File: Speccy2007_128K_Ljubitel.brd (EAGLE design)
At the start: 168.6 x 112.4 mm, 114 parts, among them X1 5V, X2 SCART-F, X3 PS/2 KB, X4 SD Card, X5 ByteBlaster, X6 AVRISP

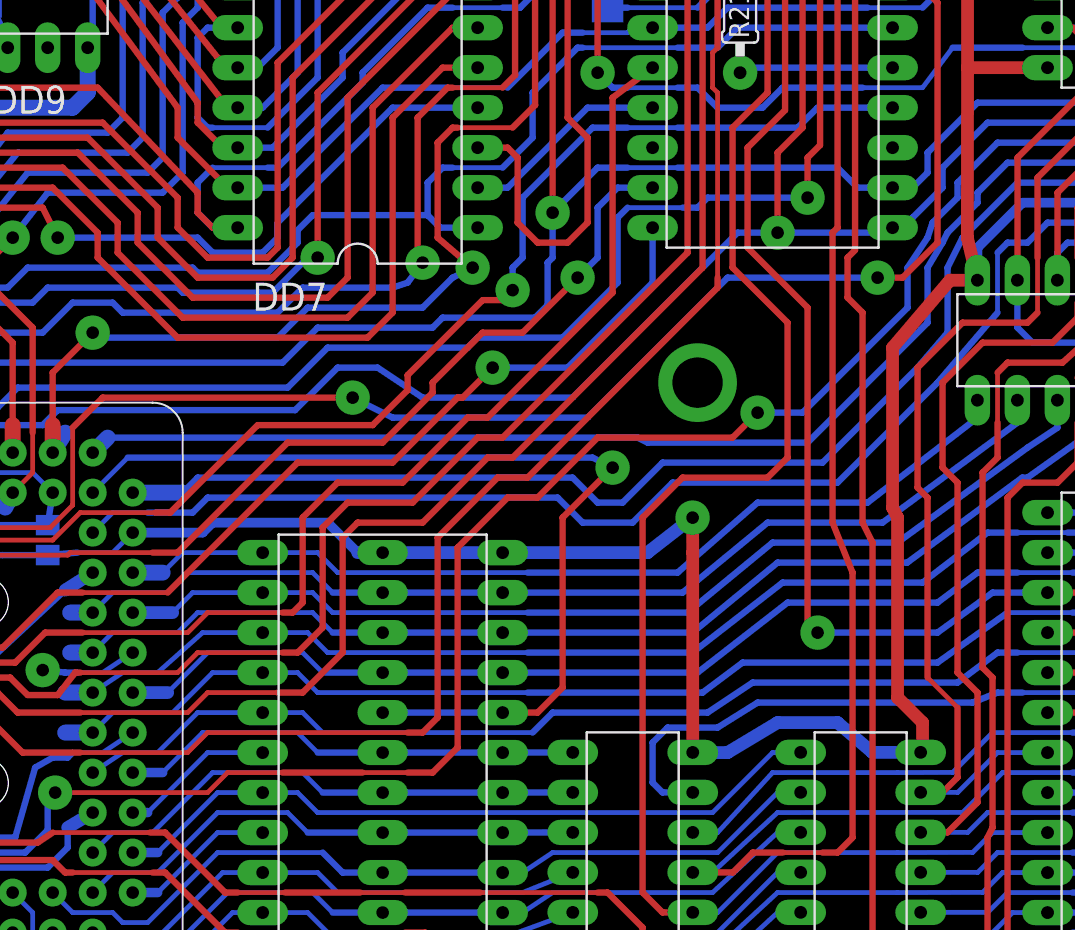
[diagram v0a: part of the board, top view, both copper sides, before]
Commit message: .
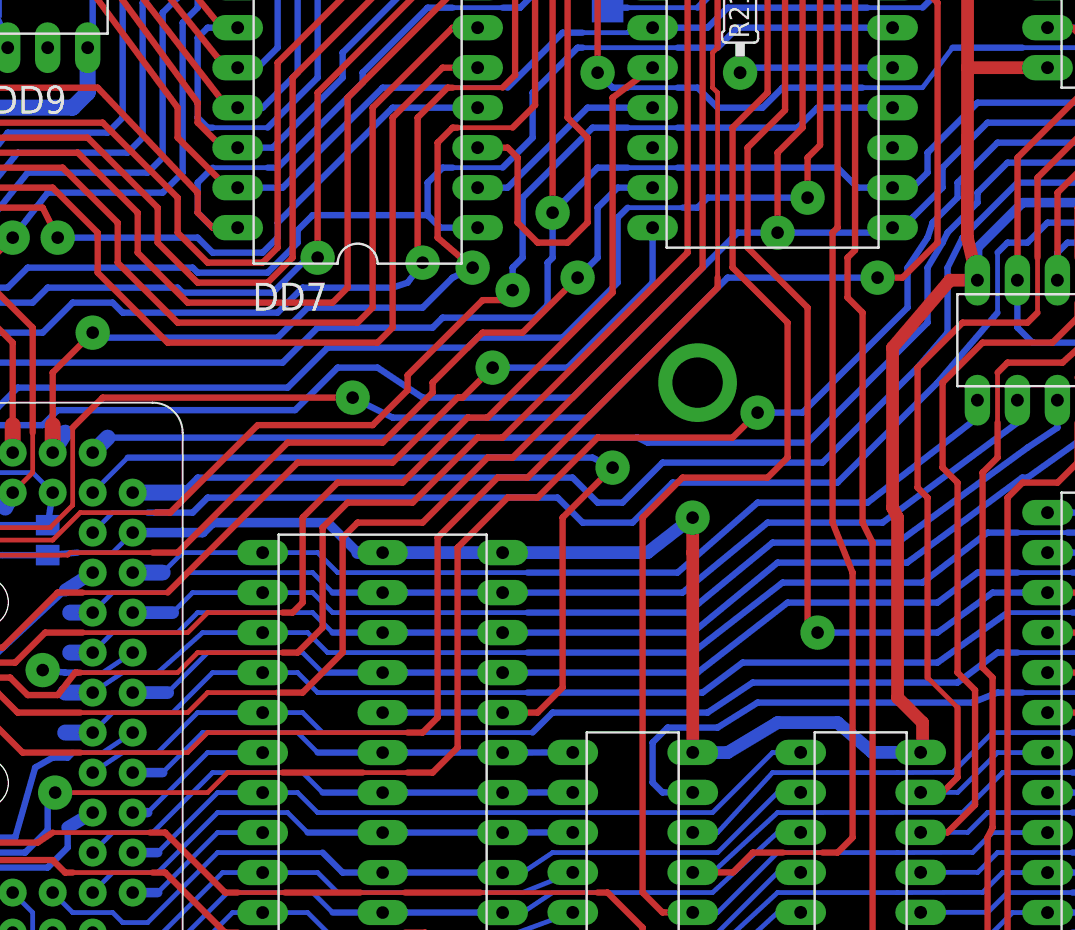
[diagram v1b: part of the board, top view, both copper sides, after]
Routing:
- net SDC: track 111.1 -> 112.5 mm
- net MOSI: track 127.0 -> 128.2 mm
- net MISO: track 130.2 -> 131.2 mm
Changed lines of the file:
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@@
 <wire x1="129.8575" y1="86.83625" x2="136.525" y2="84.29625" width="0.3048" layer="16"/>
 <wire x1="136.525" y1="84.29625" x2="138.1125" y2="84.29625" width="0.3048" layer="16"/>
-<wire x1="133.6675" y1="31.90875" x2="133.6675" y2="24.93625" width="0.4064" layer="1"/>
-<wire x1="133.6675" y1="24.93625" x2="131.7625" y2="23.03125" width="0.4064" layer="1"/>
+<wire x1="133.50875" y1="32.0675" x2="133.50875" y2="24.7775" width="0.4064" layer="1"/>
+<wire x1="133.50875" y1="24.7775" x2="131.7625" y2="23.03125" width="0.4064" layer="1"/>
 <wire x1="131.7625" y1="23.03125" x2="130.055" y2="23.03125" width="0.4064" layer="1"/>
 <wire x1="140.0175" y1="59.53125" x2="140.0175" y2="56.67375" width="0.3048" layer="1"/>
 <wire x1="131.445" y1="46.19625" x2="132.3975" y2="45.24375" width="0.4064" layer="1"/>
 <wire x1="132.3975" y1="45.24375" x2="132.3975" y2="33.17875" width="0.4064" layer="1"/>
-<wire x1="132.3975" y1="33.17875" x2="133.6675" y2="31.90875" width="0.4064" layer="1"/>
+<wire x1="132.3975" y1="33.17875" x2="133.50875" y2="32.0675" width="0.4064" layer="1"/>
 <wire x1="131.445" y1="46.19625" x2="131.445" y2="51.59375" width="0.4064" layer="1"/>
 <wire x1="131.445" y1="51.59375" x2="133.985" y2="54.13375" width="0.4064" layer="1"/>
@@
 <wire x1="100.965" y1="81.75625" x2="100.33" y2="82.39125" width="0.4064" layer="1"/>
 <wire x1="100.33" y1="82.39125" x2="99.695" y2="83.66125" width="0.4064" layer="1"/>
-<wire x1="89.2175" y1="60.16625" x2="88.5825" y2="59.53125" width="0.4064" layer="1"/>
-<wire x1="88.5825" y1="59.53125" x2="84.7725" y2="59.53125" width="0.4064" layer="1"/>
-<wire x1="84.7725" y1="59.53125" x2="82.8675" y2="61.43625" width="0.4064" layer="1"/>
-<wire x1="82.8675" y1="61.43625" x2="82.8675" y2="63.34125" width="0.4064" layer="1"/>
+<wire x1="89.2175" y1="60.16625" x2="88.265" y2="59.21375" width="0.4064" layer="1"/>
+<wire x1="88.265" y1="59.21375" x2="84.7725" y2="59.21375" width="0.4064" layer="1"/>
+<wire x1="84.7725" y1="59.21375" x2="82.8675" y2="61.11875" width="0.4064" layer="1"/>
+<wire x1="82.8675" y1="61.11875" x2="82.8675" y2="63.34125" width="0.4064" layer="1"/>
 <wire x1="82.8675" y1="63.34125" x2="78.105" y2="68.10375" width="0.4064" layer="1"/>
 <wire x1="78.105" y1="68.10375" x2="47.3075" y2="68.10375" width="0.4064" layer="1"/>
@@
 <wire x1="101.9175" y1="71.59625" x2="99.695" y2="71.59625" width="0.4064" layer="1"/>
 <wire x1="99.695" y1="71.59625" x2="96.52" y2="68.42125" width="0.4064" layer="1"/>
-<wire x1="96.52" y1="68.42125" x2="96.52" y2="56.03875" width="0.4064" layer="1"/>
-<wire x1="96.52" y1="56.03875" x2="94.9325" y2="54.45125" width="0.4064" layer="1"/>
-<wire x1="94.9325" y1="54.45125" x2="82.8675" y2="54.45125" width="0.4064" layer="1"/>
-<wire x1="82.8675" y1="54.45125" x2="77.7875" y2="59.53125" width="0.4064" layer="1"/>
-<wire x1="77.7875" y1="59.53125" x2="77.7875" y2="61.11875" width="0.4064" layer="1"/>
+<wire x1="96.52" y1="68.42125" x2="96.52" y2="55.08625" width="0.4064" layer="1"/>
+<wire x1="96.52" y1="55.08625" x2="95.5675" y2="54.13375" width="0.4064" layer="1"/>
+<wire x1="95.5675" y1="54.13375" x2="82.2325" y2="54.13375" width="0.4064" layer="1"/>
+<wire x1="82.2325" y1="54.13375" x2="77.7875" y2="58.57875" width="0.4064" layer="1"/>
+<wire x1="77.7875" y1="58.57875" x2="77.7875" y2="61.11875" width="0.4064" layer="1"/>
 <wire x1="77.7875" y1="61.11875" x2="74.93" y2="63.97625" width="0.4064" layer="1"/>
 <wire x1="74.93" y1="63.97625" x2="49.53" y2="63.97625" width="0.4064" layer="1"/>
@@
 <wire x1="101.9175" y1="74.13625" x2="100.33" y2="74.13625" width="0.4064" layer="1"/>
 <wire x1="100.33" y1="74.13625" x2="95.25" y2="69.05625" width="0.4064" layer="1"/>
-<wire x1="95.25" y1="69.05625" x2="95.25" y2="57.30875" width="0.4064" layer="1"/>
-<wire x1="95.25" y1="57.30875" x2="93.6625" y2="55.72125" width="0.4064" layer="1"/>
-<wire x1="93.6625" y1="55.72125" x2="83.185" y2="55.72125" width="0.4064" layer="1"/>
-<wire x1="83.185" y1="55.72125" x2="79.0575" y2="59.84875" width="0.4064" layer="1"/>
-<wire x1="79.0575" y1="59.84875" x2="79.0575" y2="61.75375" width="0.4064" layer="1"/>
+<wire x1="95.25" y1="69.05625" x2="95.25" y2="56.35625" width="0.4064" layer="1"/>
+<wire x1="95.25" y1="56.35625" x2="94.2975" y2="55.40375" width="0.4064" layer="1"/>
+<wire x1="94.2975" y1="55.40375" x2="82.8675" y2="55.40375" width="0.4064" layer="1"/>
+<wire x1="82.8675" y1="55.40375" x2="79.0575" y2="59.21375" width="0.4064" layer="1"/>
+<wire x1="79.0575" y1="59.21375" x2="79.0575" y2="61.75375" width="0.4064" layer="1"/>
 <wire x1="79.0575" y1="61.75375" x2="75.565" y2="65.24625" width="0.4064" layer="1"/>
 <wire x1="75.565" y1="65.24625" x2="49.2125" y2="65.24625" width="0.4064" layer="1"/>
@@
 <wire x1="101.9175" y1="76.67625" x2="100.6475" y2="76.67625" width="0.4064" layer="1"/>
 <wire x1="100.6475" y1="76.67625" x2="93.6625" y2="69.69125" width="0.4064" layer="1"/>
-<wire x1="93.6625" y1="69.69125" x2="93.6625" y2="58.26125" width="0.4064" layer="1"/>
+<wire x1="93.6625" y1="69.69125" x2="93.6625" y2="57.62625" width="0.4064" layer="1"/>
 <wire x1="76.5175" y1="66.19875" x2="80.3275" y2="62.38875" width="0.4064" layer="1"/>
-<wire x1="80.3275" y1="62.38875" x2="80.3275" y2="60.48375" width="0.4064" layer="1"/>
-<wire x1="80.3275" y1="60.48375" x2="83.82" y2="56.99125" width="0.4064" layer="1"/>
-<wire x1="83.82" y1="56.99125" x2="92.3925" y2="56.99125" width="0.4064" layer="1"/>
-<wire x1="92.3925" y1="56.99125" x2="93.6625" y2="58.26125" width="0.4064" layer="1"/>
+<wire x1="80.3275" y1="62.38875" x2="80.3275" y2="59.84875" width="0.4064" layer="1"/>
+<wire x1="80.3275" y1="59.84875" x2="83.5025" y2="56.67375" width="0.4064" layer="1"/>
+<wire x1="83.5025" y1="56.67375" x2="92.71" y2="56.67375" width="0.4064" layer="1"/>
+<wire x1="92.71" y1="56.67375" x2="93.6625" y2="57.62625" width="0.4064" layer="1"/>
 <wire x1="76.5175" y1="66.19875" x2="48.5775" y2="66.19875" width="0.4064" layer="1"/>
 <via x="19.84375" y="37.465" extent="1-16" drill="0.8" diameter="2.1844"/>
@@
 <wire x1="97.155" y1="77.94625" x2="90.17" y2="70.96125" width="0.4064" layer="1"/>
 <wire x1="90.17" y1="70.96125" x2="90.17" y2="59.53125" width="0.4064" layer="1"/>
-<wire x1="90.17" y1="59.53125" x2="88.9" y2="58.26125" width="0.4064" layer="1"/>
-<wire x1="88.9" y1="58.26125" x2="84.1375" y2="58.26125" width="0.4064" layer="1"/>
-<wire x1="84.1375" y1="58.26125" x2="81.5975" y2="60.80125" width="0.4064" layer="1"/>
-<wire x1="81.5975" y1="60.80125" x2="81.5975" y2="62.70625" width="0.4064" layer="1"/>
+<wire x1="90.17" y1="59.53125" x2="88.5825" y2="57.94375" width="0.4064" layer="1"/>
+<wire x1="88.5825" y1="57.94375" x2="84.1375" y2="57.94375" width="0.4064" layer="1"/>
+<wire x1="84.1375" y1="57.94375" x2="81.5975" y2="60.48375" width="0.4064" layer="1"/>
+<wire x1="81.5975" y1="60.48375" x2="81.5975" y2="62.70625" width="0.4064" layer="1"/>
 <wire x1="81.5975" y1="62.70625" x2="77.1525" y2="67.15125" width="0.4064" layer="1"/>
 <wire x1="77.1525" y1="67.15125" x2="47.9425" y2="67.15125" width="0.4064" layer="1"/>
